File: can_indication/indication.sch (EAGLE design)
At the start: 1 part

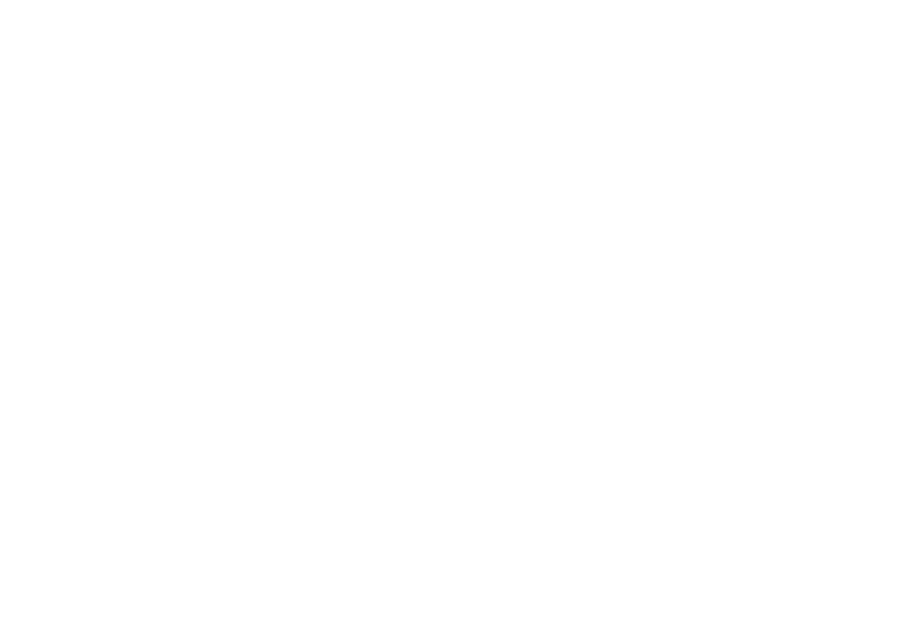
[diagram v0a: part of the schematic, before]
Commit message: Added Cree RGB LED and PCA9685 to library.
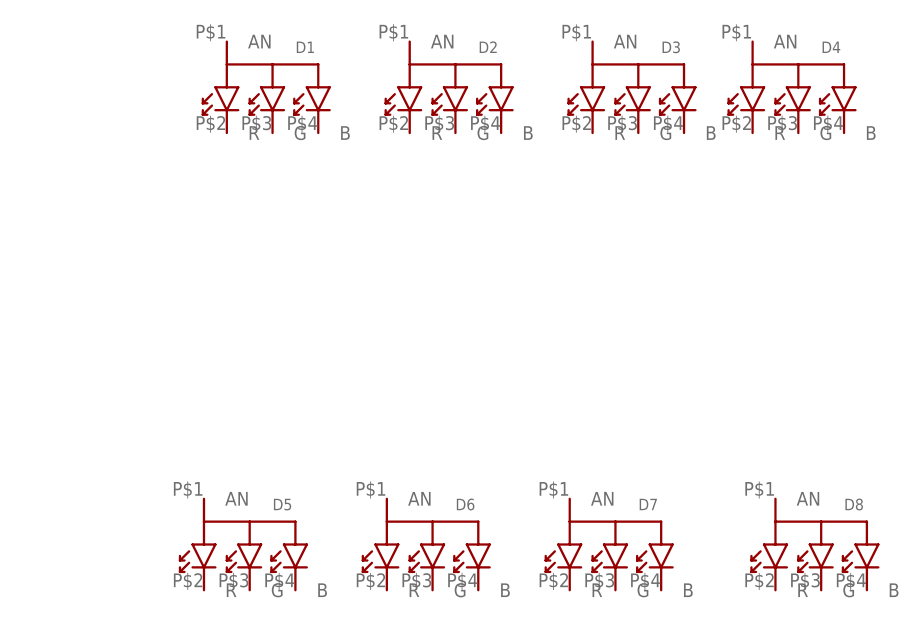
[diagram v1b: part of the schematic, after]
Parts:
- added D1, D2, D3, D4, D5, D6, D7, D8: CLV1L-FKB-CHMMQEHBB7673673, SPEAR:CLV1L-FKB-CHMMQEHBB7673673
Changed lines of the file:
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@@
 <parts>
 <part name="U$1" library="SPEAR" deviceset="MCP2562-E/SN" device=""/>
+<part name="D1" library="SPEAR" deviceset="CLV1L-FKB-CHMMQEHBB7673673" device=""/>
+<part name="D2" library="SPEAR" deviceset="CLV1L-FKB-CHMMQEHBB7673673" device=""/>
+<part name="D3" library="SPEAR" deviceset="CLV1L-FKB-CHMMQEHBB7673673" device=""/>
+<part name="D4" library="SPEAR" deviceset="CLV1L-FKB-CHMMQEHBB7673673" device=""/>
+<part name="D5" library="SPEAR" deviceset="CLV1L-FKB-CHMMQEHBB7673673" device=""/>
+<part name="D6" library="SPEAR" deviceset="CLV1L-FKB-CHMMQEHBB7673673" device=""/>
+<part name="D7" library="SPEAR" deviceset="CLV1L-FKB-CHMMQEHBB7673673" device=""/>
+<part name="D8" library="SPEAR" deviceset="CLV1L-FKB-CHMMQEHBB7673673" device=""/>
 </parts>
 <sheets>
@@
 <instances>
 <instance part="U$1" gate="G$1" x="10.16" y="-5.08"/>
+<instance part="D1" gate="G$1" x="116.84" y="33.02"/>
+<instance part="D2" gate="G$1" x="137.16" y="33.02"/>
+<instance part="D3" gate="G$1" x="157.48" y="33.02"/>
+<instance part="D4" gate="G$1" x="175.26" y="33.02"/>
+<instance part="D5" gate="G$1" x="114.3" y="-17.78"/>
+<instance part="D6" gate="G$1" x="134.62" y="-17.78"/>
+<instance part="D7" gate="G$1" x="154.94" y="-17.78"/>
+<instance part="D8" gate="G$1" x="177.8" y="-17.78"/>
 </instances>
 <busses>

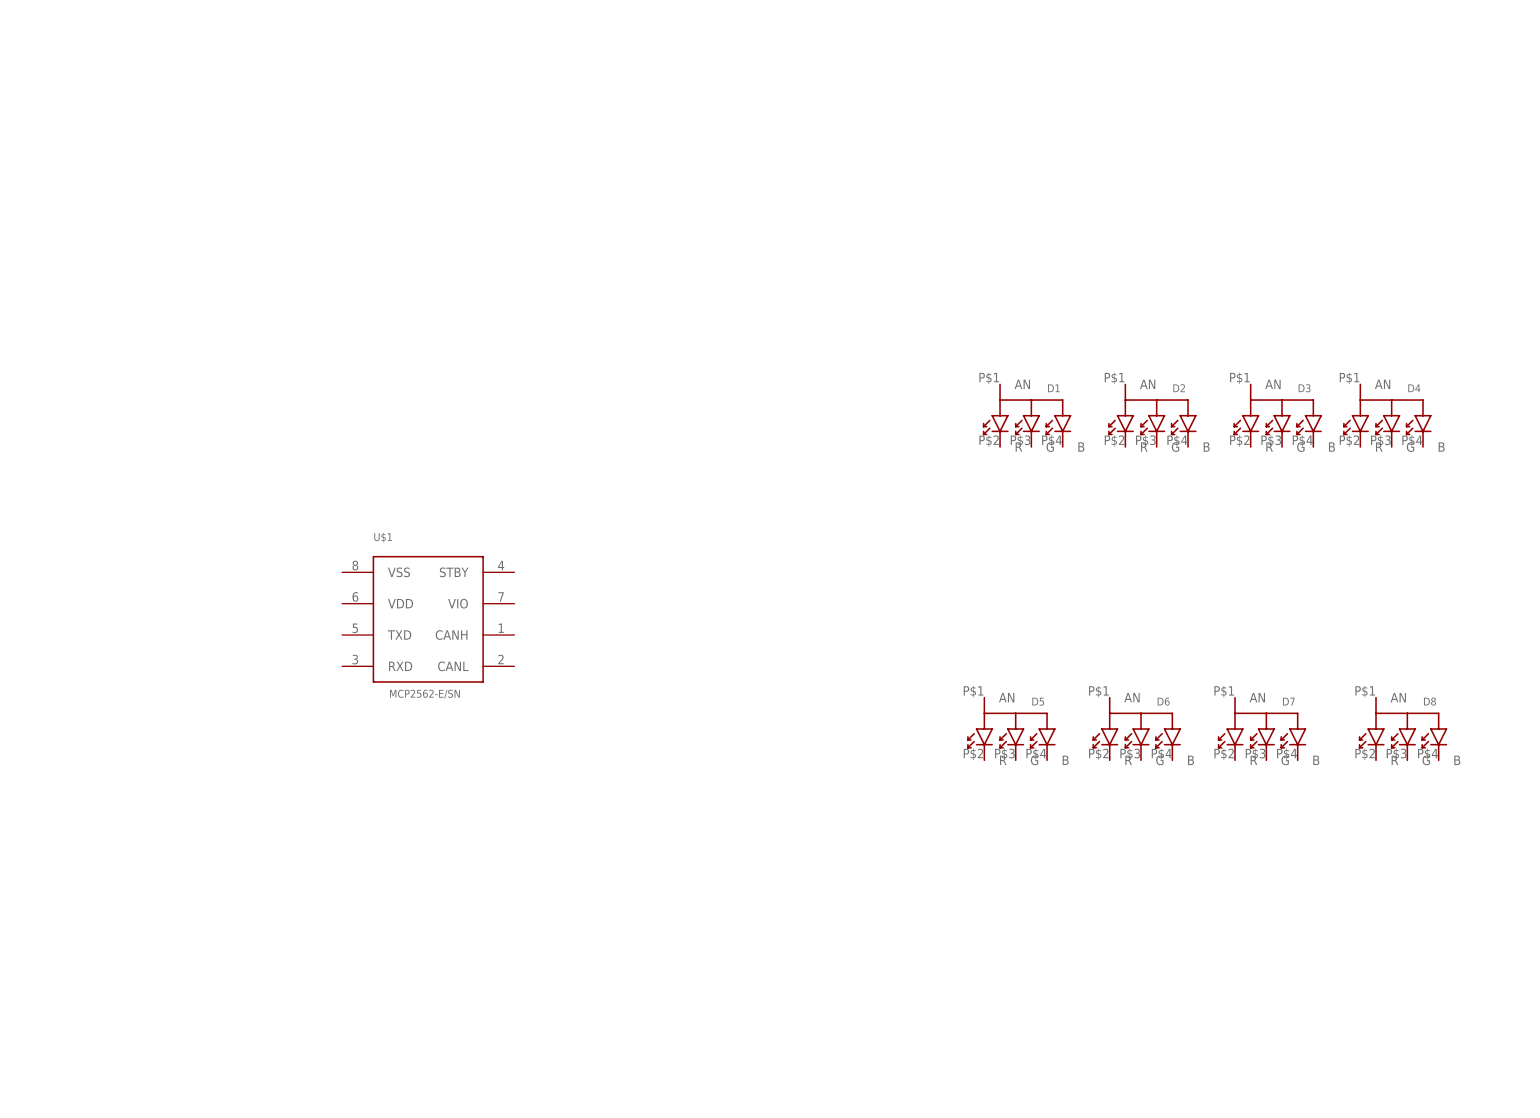
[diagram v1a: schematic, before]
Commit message: Added STM32F103CB device.
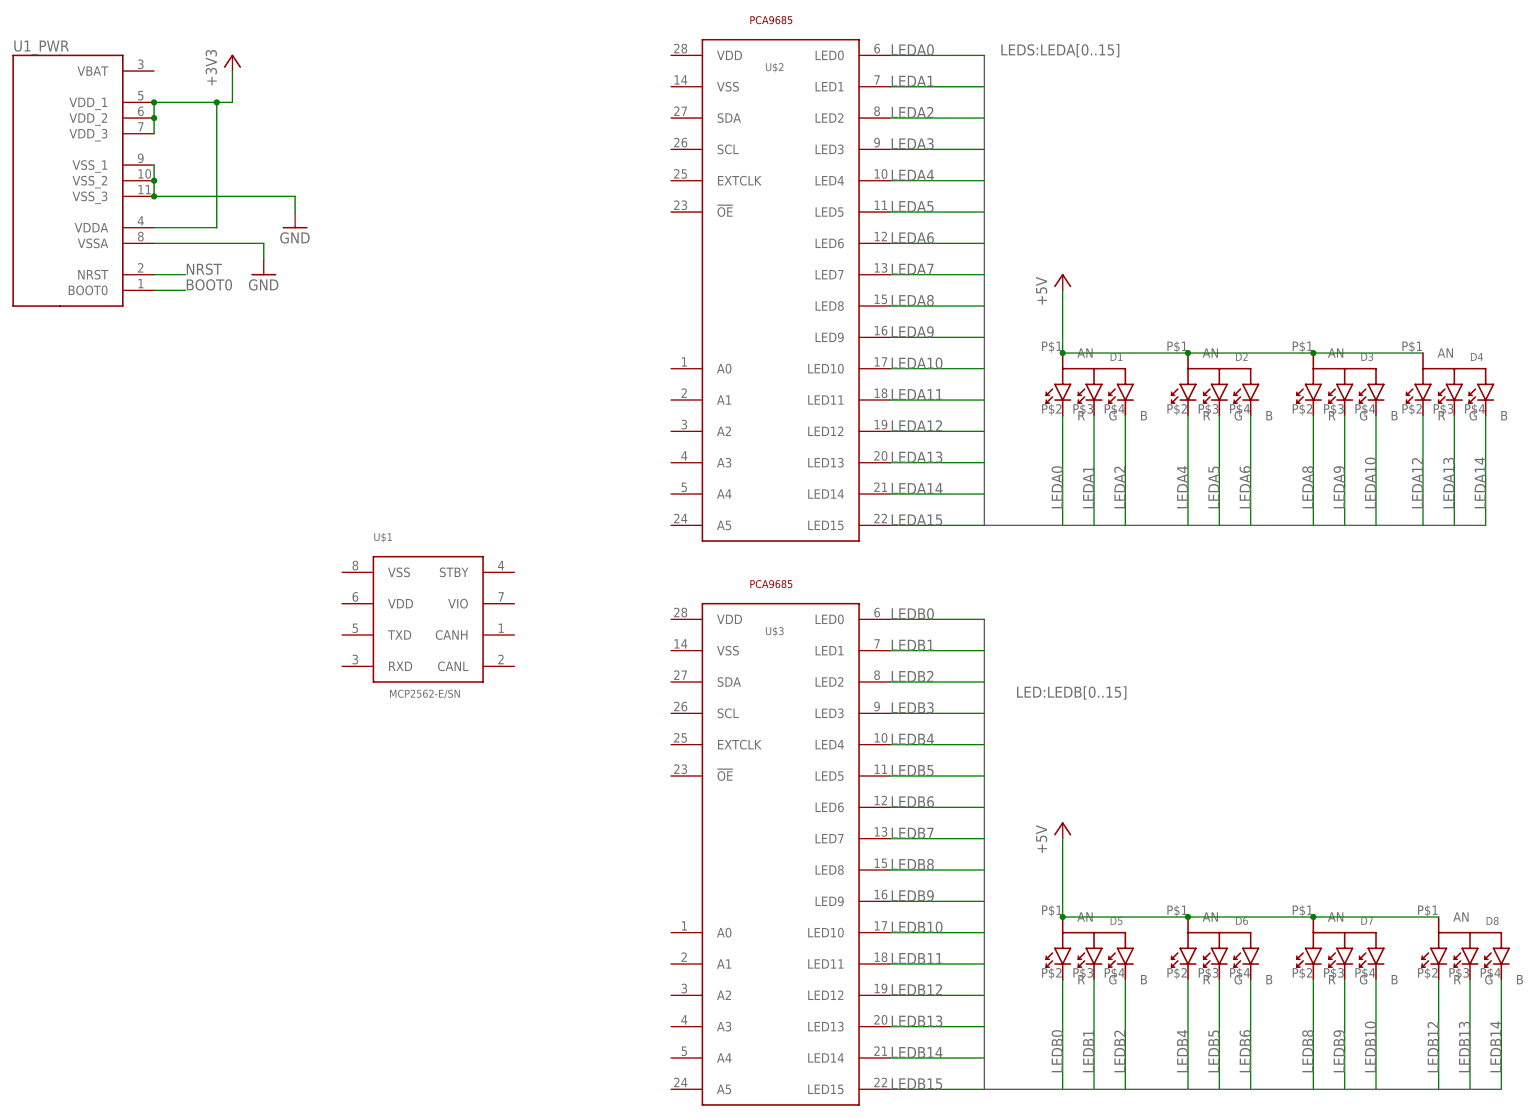
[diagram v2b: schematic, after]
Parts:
- added U$2, U$3: PCA9685PW, SPEAR:PCA9685PW
- added U1: STM32F103CB, SPEAR:STM32F103CB
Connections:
- new net +3V3: U1_PWR.VDDA, U1_PWR.VDD_1, U1_PWR.VDD_2, U1_PWR.VDD_3
- new net +5V: D1.AN, D2.AN, D3.AN, D4.AN, D5.AN, D6.AN, D7.AN, D8.AN
- new net BOOT0: U1_PWR.BOOT0
- new net GND: U1_PWR.VSSA, U1_PWR.VSS_1, U1_PWR.VSS_2, U1_PWR.VSS_3
- new net LEDA0: D1.R, U$2.LED0
- new net LEDA1: D1.G, U$2.LED1
- new net LEDA10: D3.B, U$2.LED10
- new net LEDA11: U$2.LED11
- new net LEDA12: D4.R, U$2.LED12
- new net LEDA13: D4.G, U$2.LED13
- new net LEDA14: D4.B, U$2.LED14
- new net LEDA15: U$2.LED15
- new net LEDA2: D1.B, U$2.LED2
- new net LEDA3: U$2.LED3
- new net LEDA4: D2.R, U$2.LED4
- new net LEDA5: D2.G, U$2.LED5
- new net LEDA6: D2.B, U$2.LED6
- new net LEDA7: U$2.LED7
- new net LEDA8: D3.R, U$2.LED8
- new net LEDA9: D3.G, U$2.LED9
- new net LEDB0: D5.R, U$3.LED0
- new net LEDB1: D5.G, U$3.LED1
- new net LEDB10: D7.B, U$3.LED10
- new net LEDB11: U$3.LED11
- new net LEDB12: D8.R, U$3.LED12
- new net LEDB13: D8.G, U$3.LED13
- new net LEDB14: D8.B, U$3.LED14
- new net LEDB15: U$3.LED15
- new net LEDB2: D5.B, U$3.LED2
- new net LEDB3: U$3.LED3
- new net LEDB4: D6.R, U$3.LED4
- new net LEDB5: D6.G, U$3.LED5
- new net LEDB6: D6.B, U$3.LED6
- new net LEDB7: U$3.LED7
- new net LEDB8: D7.R, U$3.LED8
- new net LEDB9: D7.G, U$3.LED9
- new net NRST: U1_PWR.NRST
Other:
- moved on the sheet: D1, D2, D3, D4, D5, D6, D7, D8
